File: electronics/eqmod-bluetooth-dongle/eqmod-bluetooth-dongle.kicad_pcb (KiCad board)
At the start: 2 copper layers, 45.2 x 23.6 mm, 6 parts, among them J1 Mount

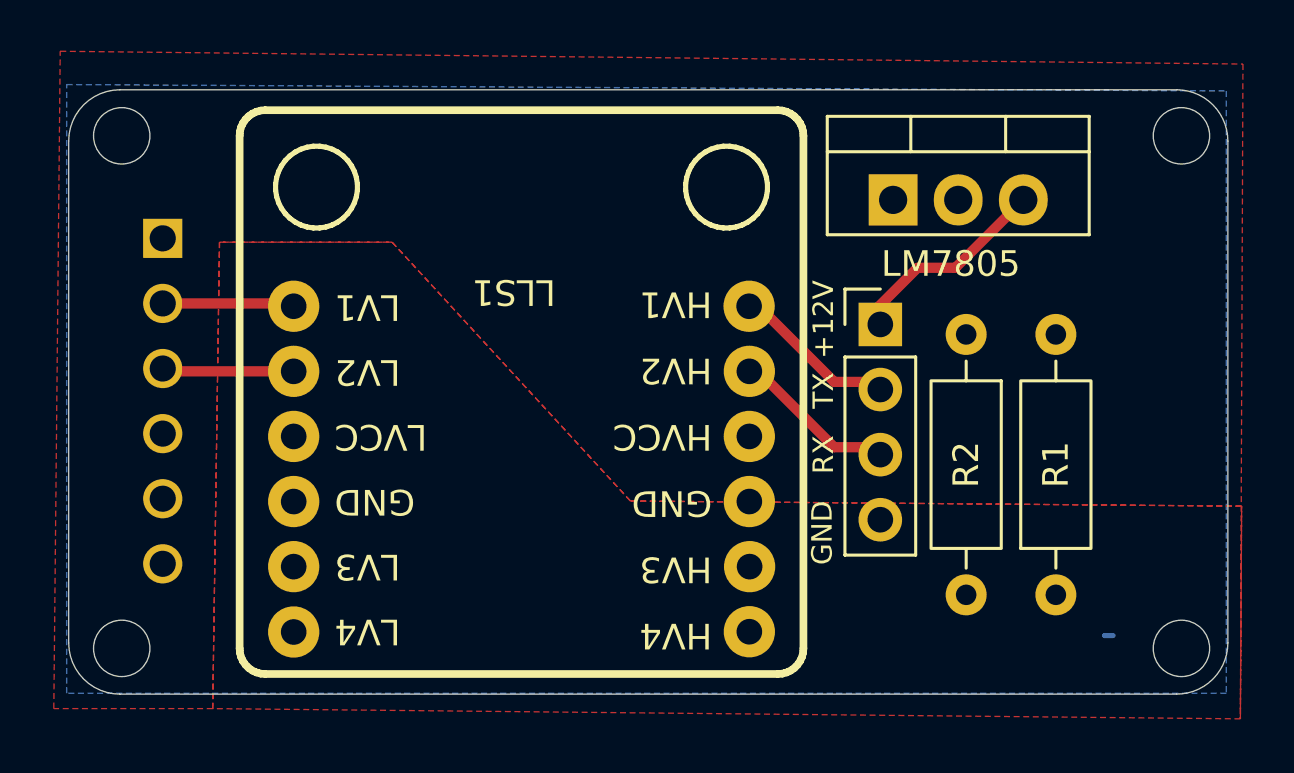
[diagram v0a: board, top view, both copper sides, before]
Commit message: With markings - ready to test
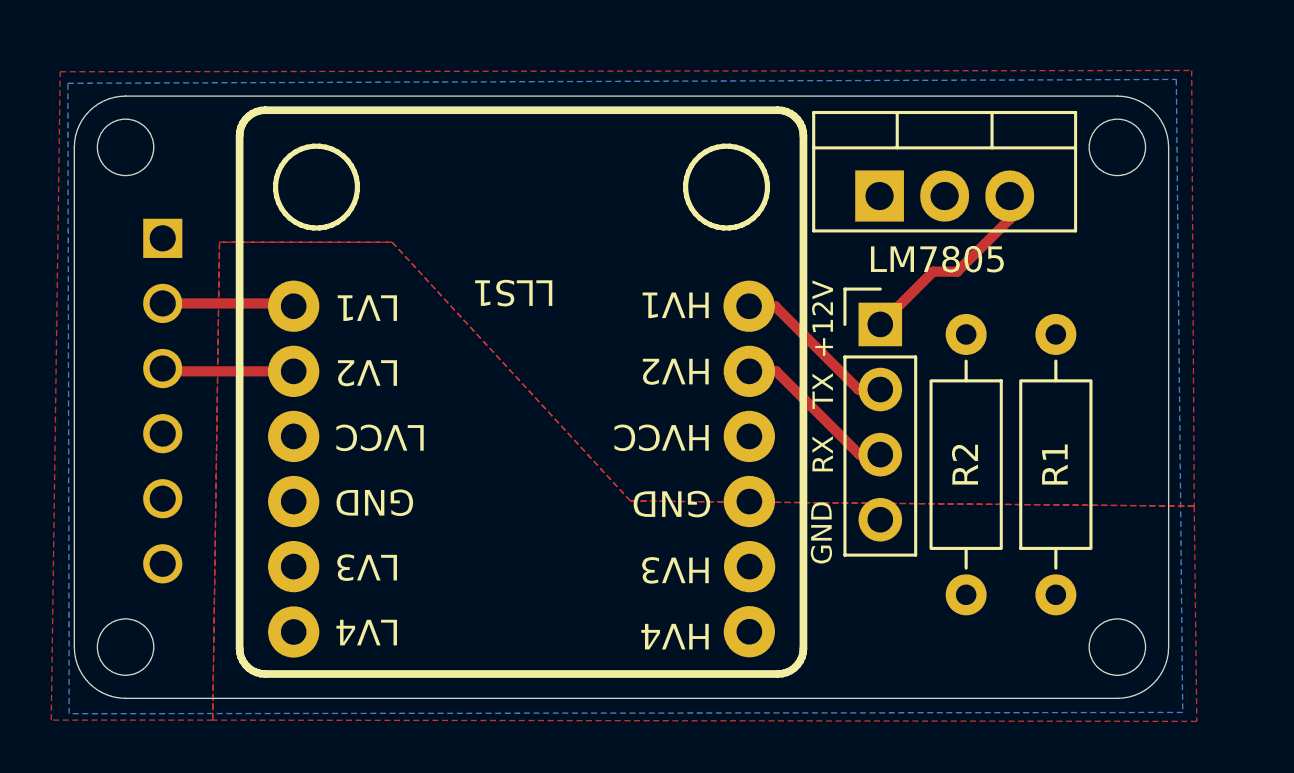
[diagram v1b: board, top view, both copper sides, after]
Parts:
- moved LM7805 0.55 mm to (137.5, 86.8)
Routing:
- net MOUNT_TX: track 5.97 -> 7.02 mm
- net MOUNT_+12V: track 8.42 -> 7.74 mm
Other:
- board size 45.2 x 23.6 mm -> 42.7 x 23.5 mm
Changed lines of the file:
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@@
 	(footprint "Package_TO_SOT_THT:TO-220-3_Vertical"
 		(layer "F.Cu")
-		(at 138 87)
+		(at 137.47 86.85)
 		(descr "TO-220-3, Vertical, RM 2.54mm, see https://www.vishay.com/docs/66542/to-220-1.pdf, generated with kicad-footprint-generator TO_SOT_THT_generate.py")
 		(tags "TO-220-3 Vertical RM 2.54mm")
@@
 		(at 109.5 94.85 180)
 		(property "Reference" "HC-05"
-			(at 2 0.1 270)
+			(at 2 0.1 90)
 			(layer "B.SilkS")
 			(effects
@@
 			(fill no)
 			(layer "B.Fab")
+		)
+		(fp_text user "TX"
+			(at -1.25 0.666666 0)
+			(unlocked yes)
+			(layer "B.SilkS")
+			(effects
+				(font
+					(size 0.8 0.8)
+					(thickness 0.1)
+				)
+				(justify right bottom mirror)
+			)
+		)
+		(fp_text user "+5V"
+			(at -1.25 -4.466667 0)
+			(unlocked yes)
+			(layer "B.SilkS")
+			(effects
+				(font
+					(size 0.8 0.8)
+					(thickness 0.1)
+				)
+				(justify right bottom mirror)
+			)
+		)
+		(fp_text user "RX"
+			(at -1.25 3.233333 0)
+			(unlocked yes)
+			(layer "B.SilkS")
+			(effects
+				(font
+					(size 0.8 0.8)
+					(thickness 0.1)
+				)
+				(justify right bottom mirror)
+			)
+		)
+		(fp_text user "GND"
+			(at -1.25 -1.9 0)
+			(unlocked yes)
+			(layer "B.SilkS")
+			(effects
+				(font
+					(size 0.8 0.8)
+					(thickness 0.1)
+				)
+				(justify right bottom mirror)
+			)
 		)
 		(pad "1" thru_hole rect
@@
 	)
 	(gr_arc
-		(start 107.83 106.284752)
-		(mid 106.415803 105.698963)
-		(end 105.83 104.284752)
+		(start 148.75 104.45)
+		(mid 148.164214 105.864214)
+		(end 146.75 106.45)
 		(stroke
 			(width 0.05)
@@
 		(layer "Edge.Cuts")
 	)
-	(gr_arc
-		(start 149.061847 82.703679)
-		(mid 150.476061 83.289465)
-		(end 151.061847 84.703679)
+	(gr_line
+		(start 108.05 82.95)
+		(end 146.75 82.95)
 		(stroke
 			(width 0.05)
@@
 		(layer "Edge.Cuts")
 	)
+	(gr_line
+		(start 106.05 104.45)
+		(end 106.05 84.95)
+		(stroke
+			(width 0.05)
+			(type default)
+		)
+		(layer "Edge.Cuts")
+	)
 	(gr_circle
-		(center 149.25 104.5)
-		(end 150.35 104.5)
+		(center 146.75 104.45)
+		(end 147.85 104.45)
 		(stroke
 			(width 0.05)
@@
 	)
 	(gr_line
-		(start 149.061847 106.284752)
-		(end 107.83 106.284752)
+		(start 146.75 106.45)
+		(end 108.05 106.45)
 		(stroke
 			(width 0.05)
@@
 	)
 	(gr_line
-		(start 151.061847 84.703679)
-		(end 151.061847 104.284752)
+		(start 148.75 84.95)
+		(end 148.75 104.45)
 		(stroke
 			(width 0.05)
@@
 		(layer "Edge.Cuts")
 	)
+	(gr_arc
+		(start 108.05 106.45)
+		(mid 106.635786 105.864214)
+		(end 106.05 104.45)
+		(stroke
+			(width 0.05)
+			(type default)
+		)
+		(layer "Edge.Cuts")
+	)
 	(gr_circle
-		(center 149.25 84.5)
-		(end 150.35 84.5)
+		(center 146.75 84.95)
+		(end 147.85 84.95)
 		(stroke
 			(width 0.05)
@@
 		(layer "Edge.Cuts")
 	)
-	(gr_line
-		(start 105.83 104.284752)
-		(end 105.83 84.703679)
+	(gr_circle
+		(center 108.05 104.45)
+		(end 109.15 104.45)
+		(stroke
+			(width 0.05)
+			(type solid)
+		)
+		(fill no)
+		(layer "Edge.Cuts")
+	)
+	(gr_arc
+		(start 106.05 84.95)
+		(mid 106.635786 83.535786)
+		(end 108.05 82.95)
 		(stroke
 			(width 0.05)
@@
 		(layer "Edge.Cuts")
 	)
-	(gr_arc
-		(start 105.83 84.703679)
-		(mid 106.415794 83.289479)
-		(end 107.83 82.703679)
-		(stroke
-			(width 0.05)
-			(type default)
-		)
-		(layer "Edge.Cuts")
-	)
 	(gr_circle
-		(center 107.9 104.5)
-		(end 109 104.5)
+		(center 108.05 84.95)
+		(end 109.15 84.95)
 		(stroke
 			(width 0.05)
@@
 		(layer "Edge.Cuts")
 	)
-	(gr_circle
-		(center 107.9 84.5)
-		(end 109 84.5)
-		(stroke
-			(width 0.05)
-			(type solid)
-		)
-		(fill no)
-		(layer "Edge.Cuts")
-	)
 	(gr_arc
-		(start 151.061847 104.284752)
-		(mid 150.476061 105.698966)
-		(end 149.061847 106.284752)
-		(stroke
-			(width 0.05)
-			(type default)
-		)
-		(layer "Edge.Cuts")
-	)
-	(gr_line
-		(start 107.83 82.703679)
-		(end 149.061847 82.703679)
+		(start 146.75 82.95)
+		(mid 148.164214 83.535786)
+		(end 148.75 84.95)
 		(stroke
 			(width 0.05)
@@
 	)
 	(segment
-		(start 139.96 87.45)
-		(end 139.91 87.5)
-		(width 0.2)
-		(layer "F.Cu")
-		(net 5)
-	)
-	(segment
 		(start 114.27 98.77)
 		(end 114.61 98.77)
@@
 	)
 	(segment
-		(start 146.25 104)
-		(end 146.58 104)
-		(width 0.2)
-		(layer "B.Cu")
-		(net 5)
-	)
-	(segment
 		(start 109.16 99)
 		(end 109.5 98.66)
@@
 	)
 	(segment
-		(start 137.04 94.1)
-		(end 135.7 94.1)
+		(start 137.46 94.4)
+		(end 137.5 94.4)
 		(width 0.4)
 		(layer "F.Cu")
@@
 	)
 	(segment
-		(start 135.7 94.1)
-		(end 132.75 91.15)
-		(width 0.4)
-		(layer "F.Cu")
-		(net 7)
-	)
-	(segment
-		(start 132.75 91.15)
+		(start 133.4 91.15)
 		(end 132.38 91.15)
 		(width 0.4)
@@
 	)
 	(segment
+		(start 137.5 94.4)
+		(end 136.65 94.4)
+		(width 0.4)
+		(layer "F.Cu")
+		(net 7)
+	)
+	(segment
+		(start 136.65 94.4)
+		(end 133.4 91.15)
+		(width 0.4)
+		(layer "F.Cu")
+		(net 7)
+	)
+	(segment
 		(start 137.1 94.04)
-		(end 137.04 94.1)
+		(end 137.46 94.4)
 		(width 0.4)
 		(layer "F.Cu")
@@
 	)
 	(segment
-		(start 137.1 91.5)
-		(end 138.95 89.65)
+		(start 137.5 91.86)
+		(end 139.56 89.8)
 		(width 0.4)
 		(layer "F.Cu")
@@
 	)
 	(segment
-		(start 138.95 89.65)
-		(end 140.43 89.65)
+		(start 142.55 87.75)
+		(end 142.55 86.85)
 		(width 0.4)
 		(layer "F.Cu")
@@
 	)
 	(segment
-		(start 143.08 87)
-		(end 143.08 87.58)
-		(width 0.2)
+		(start 140.5 89.8)
+		(end 142.55 87.75)
+		(width 0.4)
 		(layer "F.Cu")
 		(net 8)
 	)
 	(segment
-		(start 140.43 89.65)
-		(end 143.08 87)
+		(start 139.56 89.8)
+		(end 140.5 89.8)
 		(width 0.4)
 		(layer "F.Cu")
@@
 	)
 	(segment
-		(start 137.1 96.58)
-		(end 137.03 96.65)
+		(start 137.56 91.8)
+		(end 137.5 91.86)
 		(width 0.4)
 		(layer "F.Cu")
-		(net 9)
-	)
-	(segment
-		(start 135.7 96.65)
-		(end 132.74 93.69)
-		(width 0.4)
-		(layer "F.Cu")
-		(net 9)
+		(net 8)
 	)
 	(segment
@@
 	)
 	(segment
-		(start 137.03 96.65)
-		(end 135.7 96.65)
+		(start 132.39 93.69)
+		(end 133.44 93.69)
 		(width 0.4)
 		(layer "F.Cu")
@@
 	)
 	(segment
-		(start 132.81 93.69)
-		(end 132.39 93.69)
-		(width 0.2)
+		(start 133.44 93.69)
+		(end 136.69 96.94)
+		(width 0.4)
+		(layer "F.Cu")
+		(net 9)
+	)
+	(segment
+		(start 136.69 96.94)
+		(end 137.5 96.94)
+		(width 0.4)
 		(layer "F.Cu")
 		(net 9)
@@
 		(polygon
 			(pts
-				(xy 151.55 107.25) (xy 151.6 98.95) (xy 127.75 98.75) (xy 118.45 88.65) (xy 111.715231 88.65) (xy 111.45 106.85)
-				(xy 105.25 106.85) (xy 105.5 81.2) (xy 151.65 81.7)
+				(xy 149.75 98.95) (xy 149.75 98.95) (xy 127.75 98.75) (xy 118.45 88.65) (xy 111.715231 88.65) (xy 111.45 107.3)
+				(xy 105.15 107.3) (xy 105.5 82) (xy 149.65 81.95)
 			)
 		)
@@
 		(polygon
 			(pts
-				(xy 111.45 106.85) (xy 111.715231 88.65) (xy 118.45 88.65) (xy 127.75 98.75) (xy 151.6 98.95) (xy 151.55 107.25)
+				(xy 111.45 107.3) (xy 111.715231 88.65) (xy 118.45 88.65) (xy 127.75 98.75) (xy 149.75 98.95) (xy 149.85 107.35)
 			)
 		)
@@
 		(polygon
 			(pts
-				(xy 105.75 106.25) (xy 105.75 82.5) (xy 151 82.75) (xy 151 106.25)
-			)
-		)
+				(xy 105.85 107.05) (xy 105.8 82.45) (xy 149.05 82.3) (xy 149.3 107)
+			)
+		)
